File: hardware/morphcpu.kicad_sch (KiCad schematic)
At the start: 80 parts, among them J1 TYPE-C-31-M-12, SW1 TS-1187A-B-A-B, U1 ICE40UP5K-SG48I, U2 FT231XS-R, U3 W25Q32JVSSIQ, U4 AP2112K-3.3TRG1, U5 ME6211C12M5G-N, U6 USBLC6-2SC6, X1 1532H4-16000JWPDTSNL

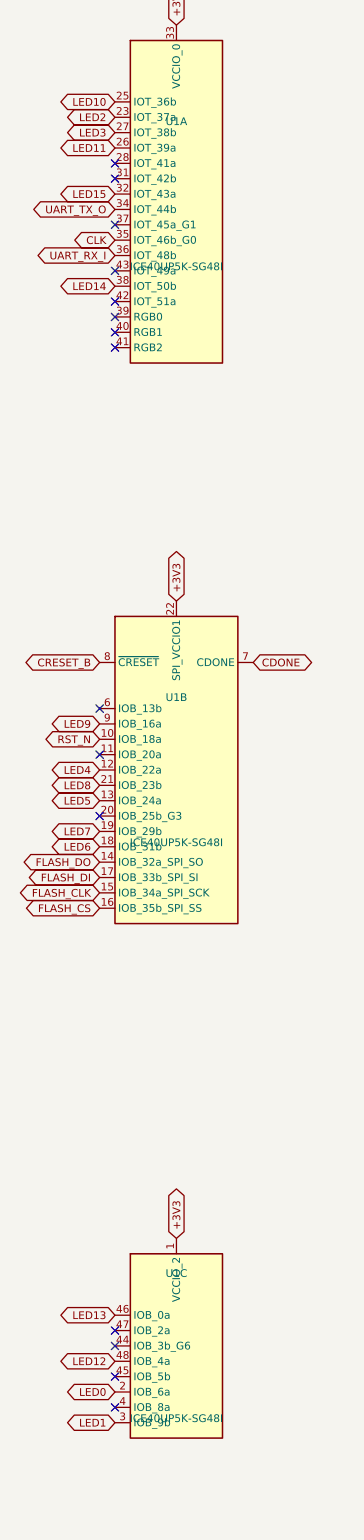
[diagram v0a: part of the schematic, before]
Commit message: 2 LEDSS!!!1!!!1!
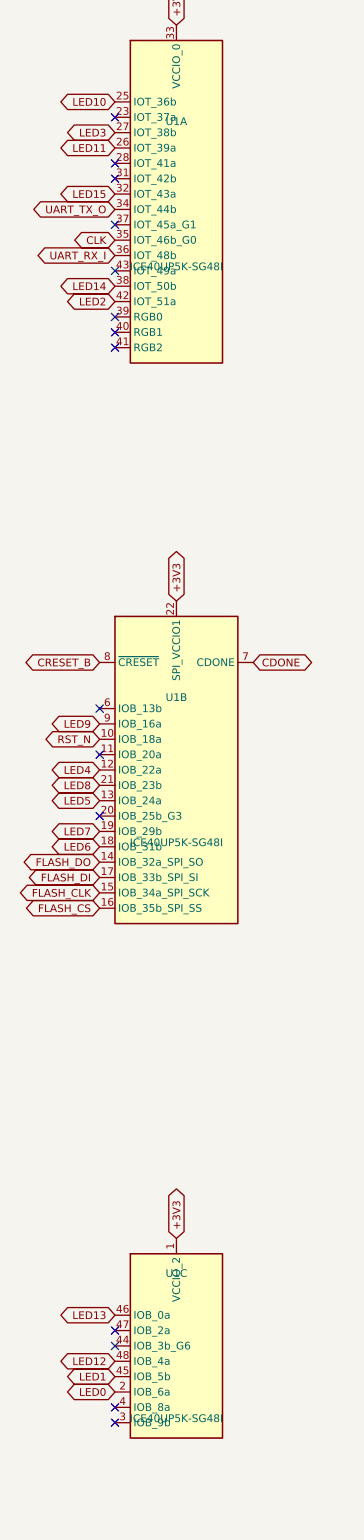
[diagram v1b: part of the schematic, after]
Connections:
- net LED1: now also U1.45 (IOB_5b); no longer U1.3 (IOB_9b)
- net LED2: now also U1.42 (IOT_51a); no longer U1.23 (IOT_37a)
